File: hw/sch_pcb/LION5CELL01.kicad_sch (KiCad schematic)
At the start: 46 parts, among them J1 USBC_USB4105-GF-A, J2 46436-9327, U2 USBLC6-2SC6, U3 FT260Q-T, U4 SHT35-DIS, U5 PCA9541ABS/01, U7 TCA4307

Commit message: wip, layout progress
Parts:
- D6, D7: footprint LED_SMD:LED_1206_3216Metric -> Mlab_D:SMD_LED_RIGHT_KINGBRIGHT_1605
- R1, R2: footprint (none) -> Resistor_SMD:R_0805_2012Metric
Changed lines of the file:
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@@
       (effects (font (size 1 1)) (justify right))
     )
-    (property "Footprint" "LED_SMD:LED_1206_3216Metric" (at 138.43 144.78 0)
+    (property "Footprint" "Mlab_D:SMD_LED_RIGHT_KINGBRIGHT_1605" (at 138.43 144.78 0)
       (effects (font (size 1 1)) hide)
     )
@@
       (effects (font (size 1.27 1.27)) (justify right))
     )
-    (property "Footprint" "" (at 52.07 64.77 0)
+    (property "Footprint" "Resistor_SMD:R_0805_2012Metric" (at 52.07 64.77 0)
       (effects (font (size 1.27 1.27)) hide)
     )
@@
       (effects (font (size 1.27 1.27)) (justify right))
     )
-    (property "Footprint" "" (at 59.69 64.77 0)
+    (property "Footprint" "Resistor_SMD:R_0805_2012Metric" (at 59.69 64.77 0)
       (effects (font (size 1.27 1.27)) hide)
     )
@@
       (effects (font (size 1 1)) (justify right))
     )
-    (property "Footprint" "LED_SMD:LED_1206_3216Metric" (at 129.54 144.78 0)
-      (effects (font (size 1 1)) hide)
-    )
+    (property "Footprint" "Mlab_D:SMD_LED_RIGHT_KINGBRIGHT_1605" (at 129.54 144.78 0)
+      (effects (font (size 1 1)) hide)
+    )

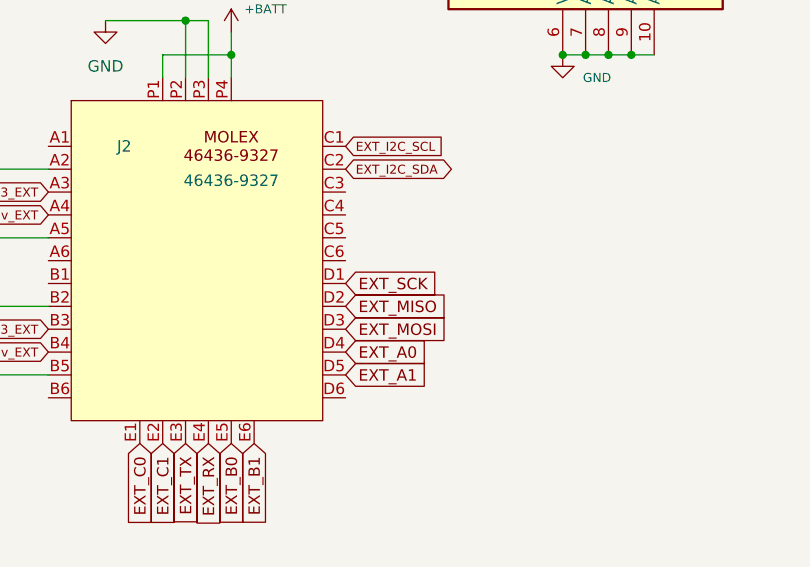
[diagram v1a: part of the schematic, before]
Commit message: wip, layout improvements
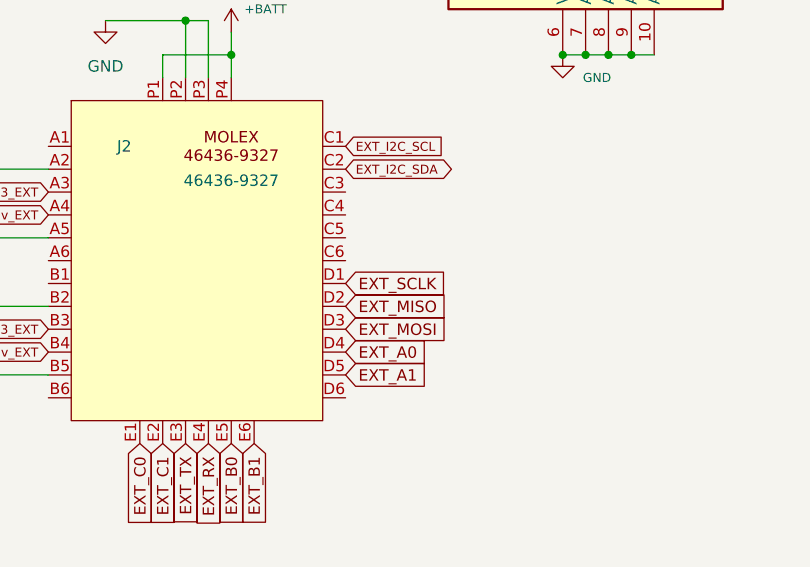
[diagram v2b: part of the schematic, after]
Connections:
- net EXT_SCK renamed EXT_SCLK
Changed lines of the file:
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@@
     )
   )
-  (global_label "EXT_SCK" (shape input) (at 212.09 132.08 0) (fields_autoplaced)
+  (global_label "EXT_SCLK" (shape input) (at 212.09 132.08 0) (fields_autoplaced)
     (effects (font (size 1.27 1.27)) (justify left))
-    (property "Intersheetrefs" "${INTERSHEET_REFS}" (at 223.1184 132.08 0)
+    (property "Intersheetrefs" "${INTERSHEET_REFS}" (at 224.1465 132.08 0)
       (effects (font (size 1.27 1.27)) (justify left) hide)
     )
